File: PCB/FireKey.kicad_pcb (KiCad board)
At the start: 2 copper layers, 99.7 x 99.1 mm, 74 parts, among them P1 Pad, P2 Pad, SW1 SW_MEC_4A, U1 Arduino_Pro_Micro_USB-C

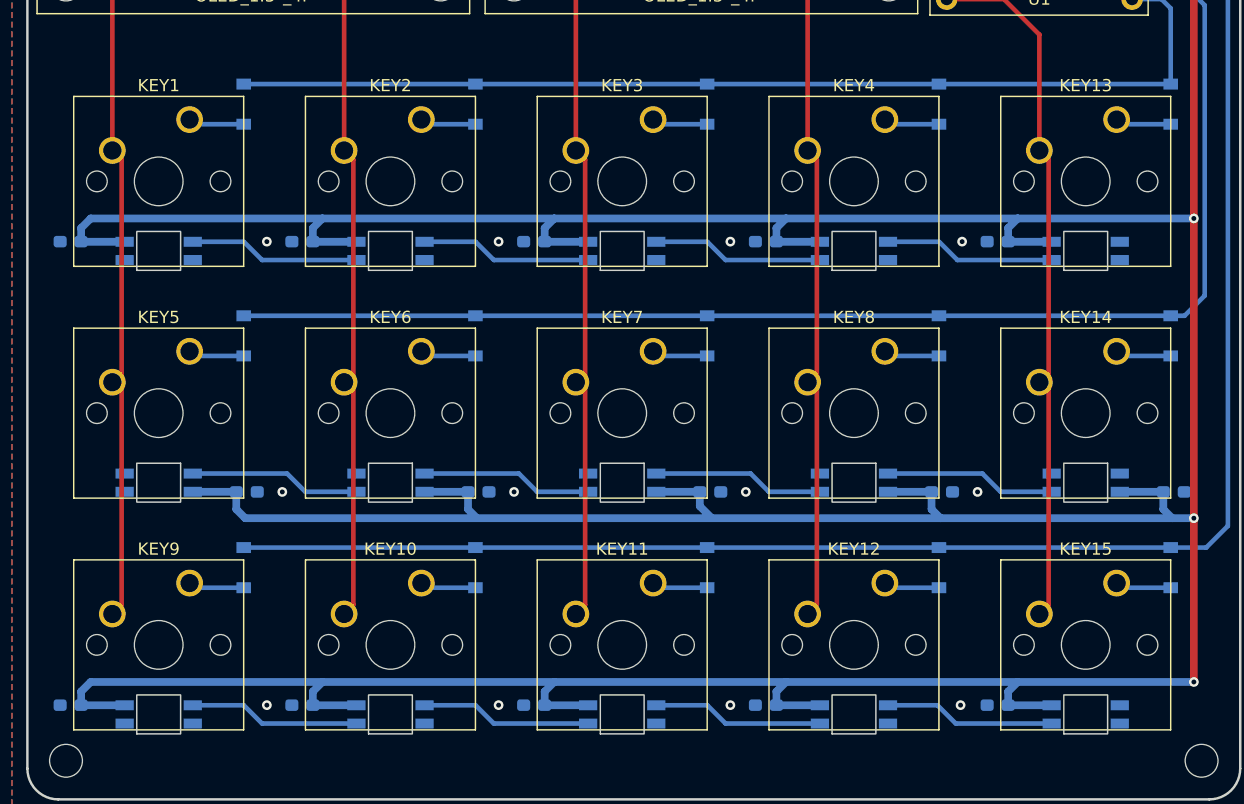
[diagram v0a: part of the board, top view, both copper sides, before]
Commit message: worked on PCB tracing and DRC errors
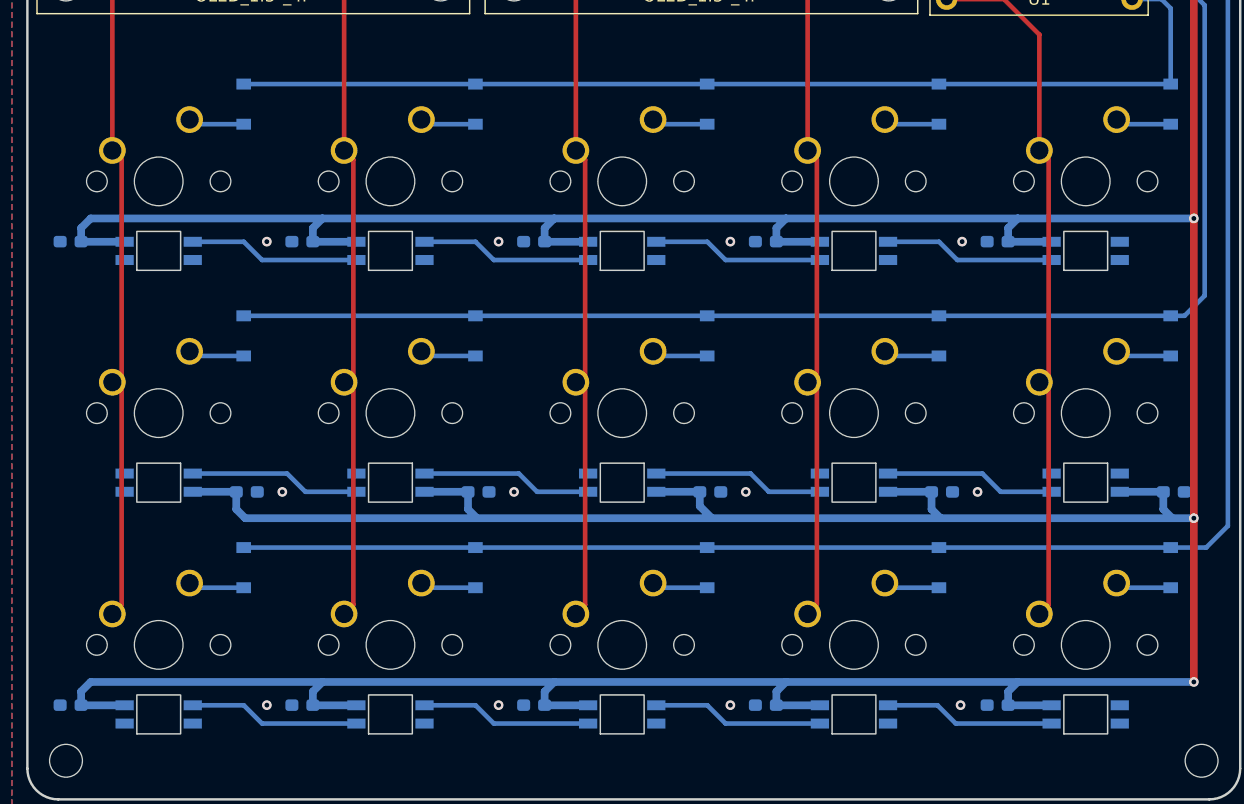
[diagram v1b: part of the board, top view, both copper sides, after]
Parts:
- KEY1, KEY10, KEY11, KEY12, KEY13, KEY14, KEY15, KEY2, KEY3, KEY4, KEY5, KEY6, KEY7, KEY8, KEY9: footprint Button_Switch_Keyboard:SW_Cherry_MX_1.00u_PCB -> Custom_Parts:SW_Cherry_MX_1.00u_PCB_CleanFront
